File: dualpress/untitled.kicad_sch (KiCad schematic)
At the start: 16 parts, among them J4 Connector, USB-TYPE-C-16P, J5 Connector, USB-TYPE-C-16P

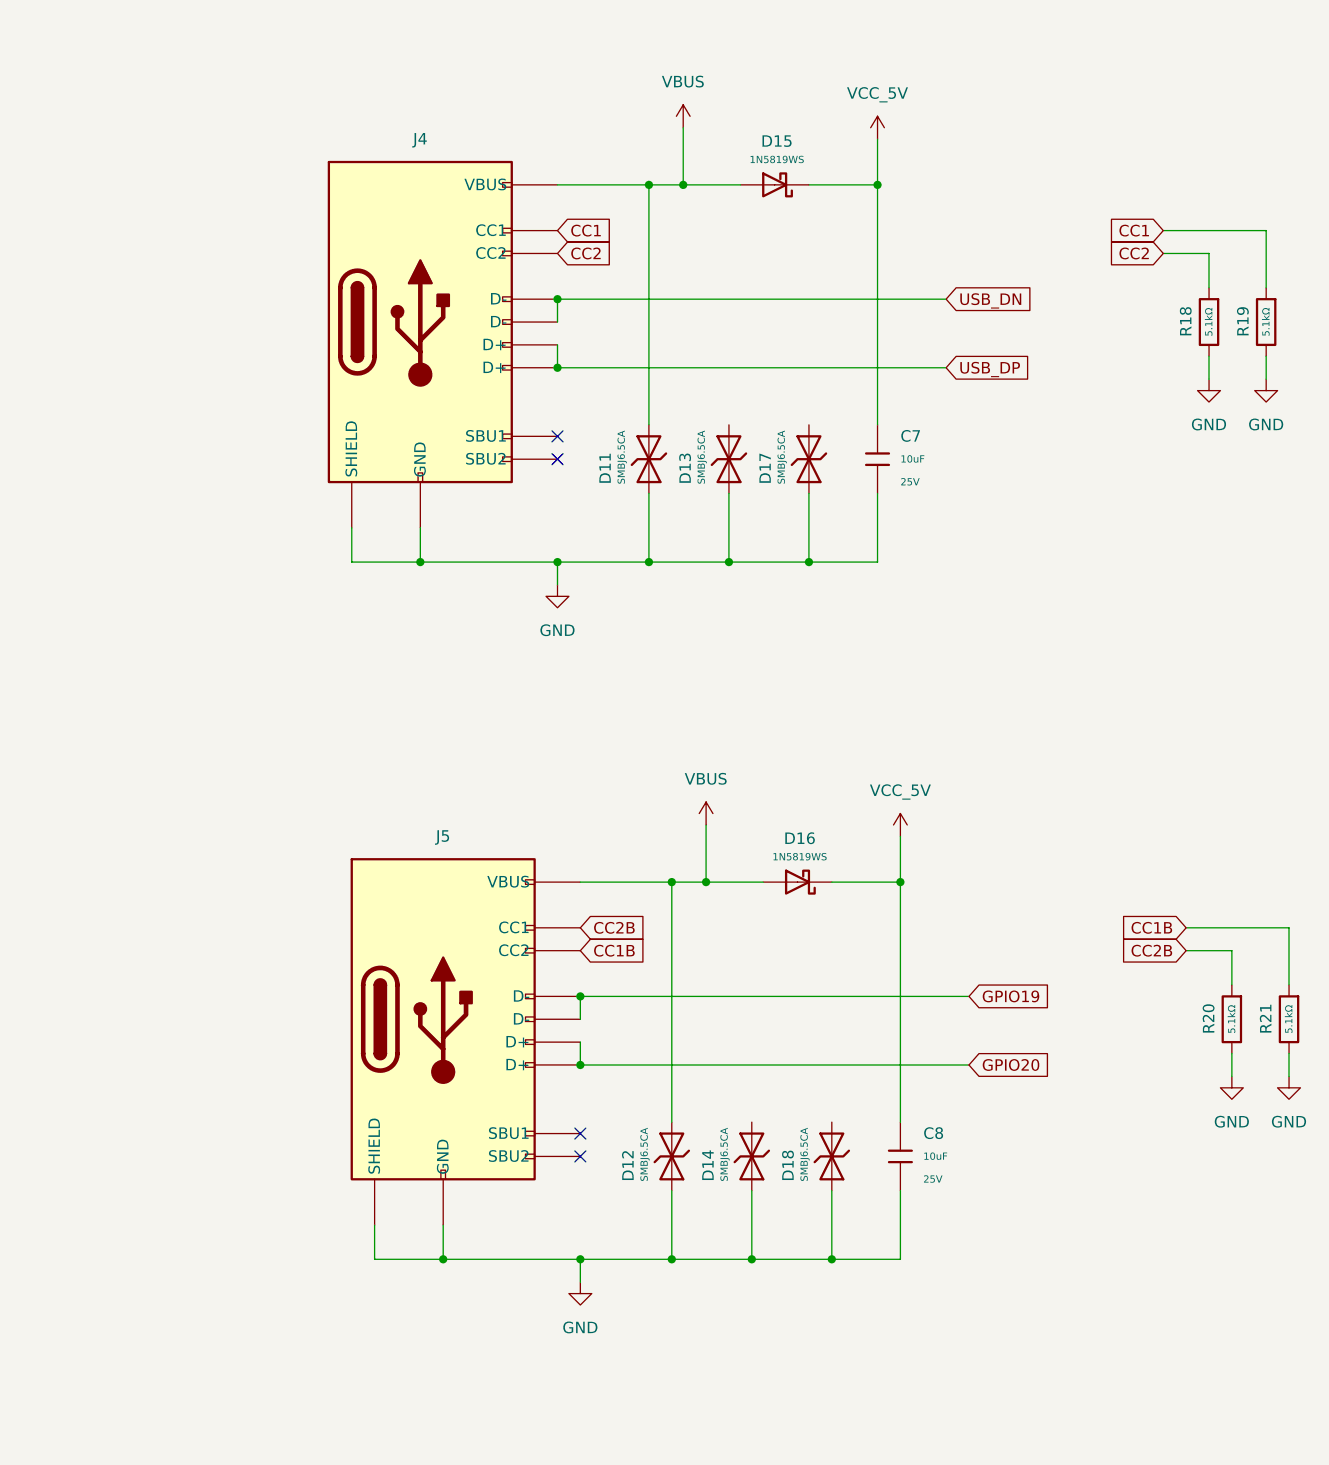
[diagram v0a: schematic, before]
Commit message: schematic done
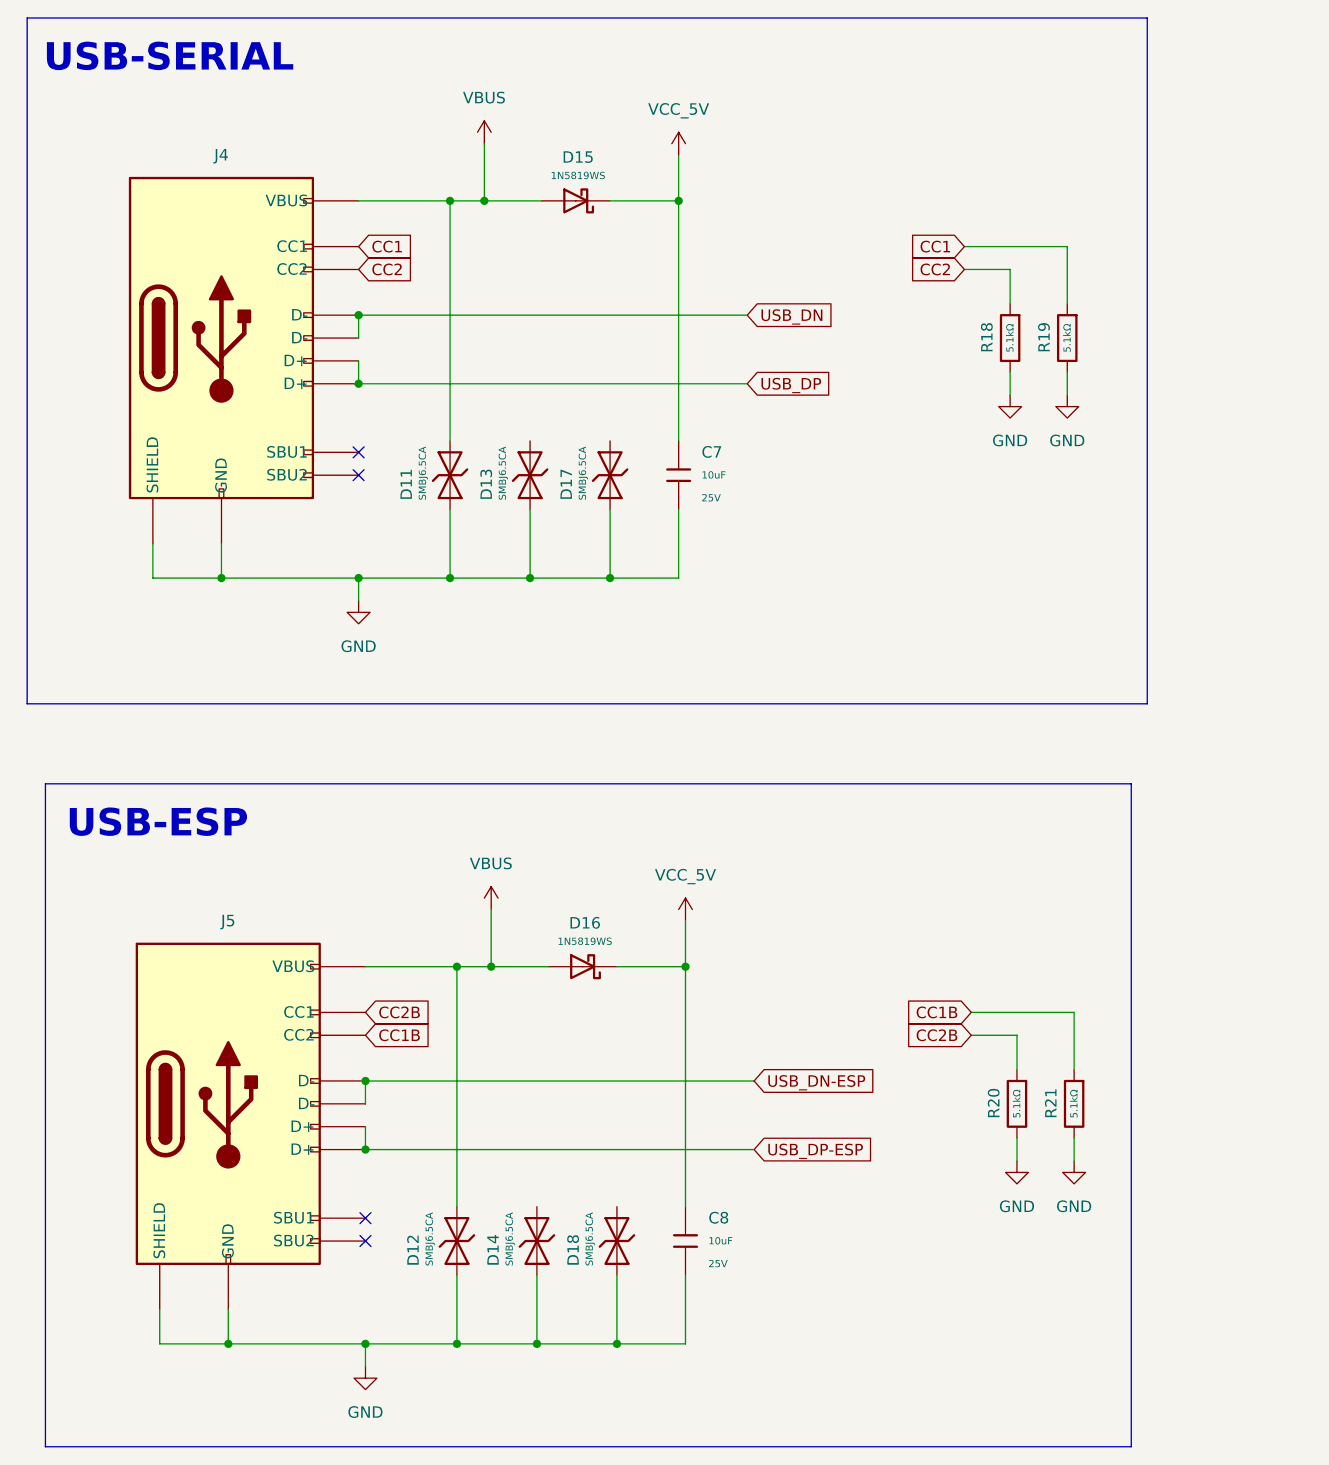
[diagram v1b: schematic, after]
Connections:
- net GPIO19 renamed USB_DN-ESP
- net GPIO20 renamed USB_DP-ESP
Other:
- note added: "USB-ESP"
- note added: "USB-SERIAL"
- moved on the sheet: C7, C8, D11, D12, D13, D14, D15, D16, D17, D18, J4, J5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

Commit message: before remove footprints
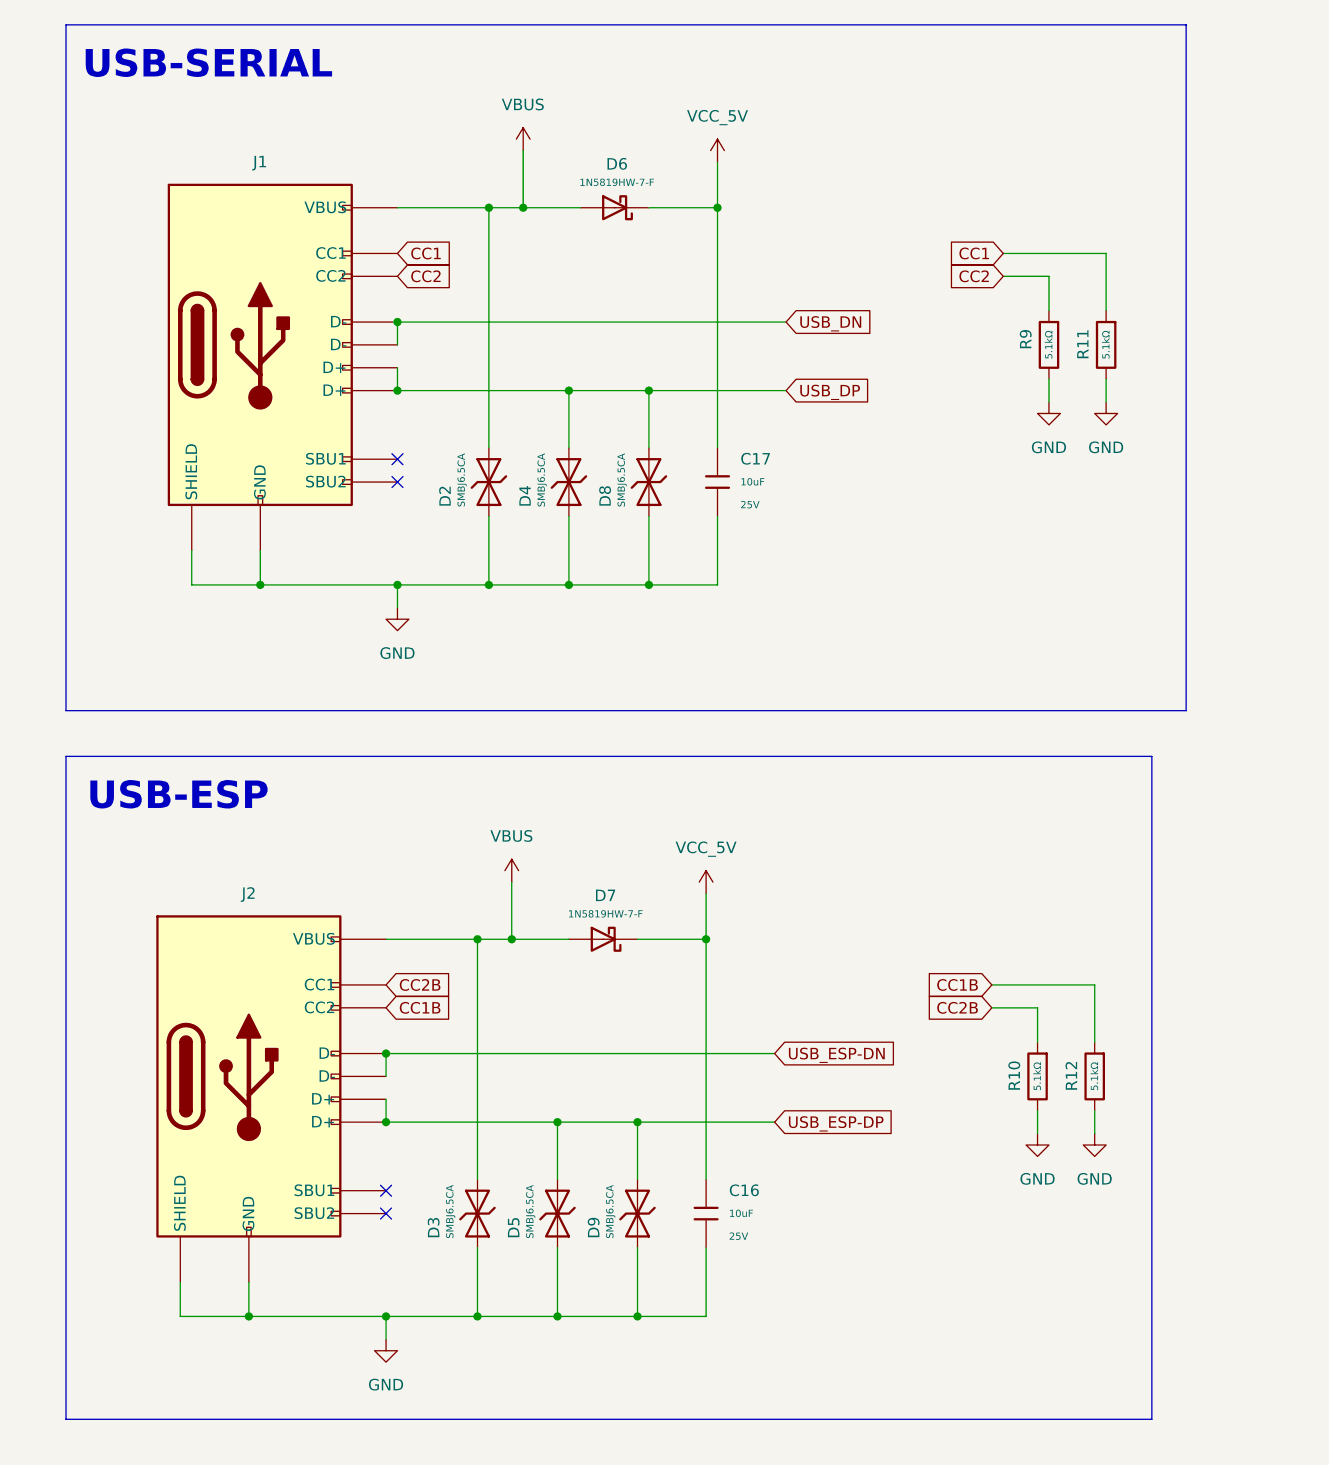
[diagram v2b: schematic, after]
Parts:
- removed C7, C8: 10uF, PCM_JLCPCB:C_0603, symbol PCM_JLCPCB-Capacitors:0603,10uF,(2)
- added C16, C17: 10uF, PCM_JLCPCB:C_0805, symbol PCM_JLCPCB-Capacitors:0805,10uF
- D2: renamed from D11; JLCPCB (none) -> C7420377
- D3: renamed from D12; JLCPCB (none) -> C7420377
- D4: renamed from D13; JLCPCB (none) -> C7420377
- D5: renamed from D14; JLCPCB (none) -> C7420377
- D6: renamed from D15; value 1N5819WS -> 1N5819HW-7-F; footprint PCM_JLCPCB:D_SOD-323 -> PCM_JLCPCB:D_SOD-123; JLCPCB (none) -> C82544; LCSC C191023 -> C82544; Part 1N5819WS -> 1N5819HW-7-F; now left out of the parts list
- D7: renamed from D16; value 1N5819WS -> 1N5819HW-7-F; footprint PCM_JLCPCB:D_SOD-323 -> PCM_JLCPCB:D_SOD-123; JLCPCB (none) -> C82544; now left out of the parts list
- D8: renamed from D17; JLCPCB (none) -> C7420377
- D9: renamed from D18; JLCPCB (none) -> C7420377
- renumbered J4 to J1, J5 to J2, R20 to R10, R19 to R11, R21 to R12, R18 to R9
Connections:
- net USB_DP-ESP is gone; now on net USB_ESP-DP: J2.A6 (D+), J2.B6 (D+)
- net GND: now also C16.2, C17.2
- net USB_DP: now also D4.2, D8.2
- net VCC_5V: now also C16.1, C17.1
- net USB_ESP-DP: now reaches D9.2
- net USB_ESP-DP: now also D5.2
- net USB_DN-ESP renamed USB_ESP-DN
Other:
- moved on the sheet: D2, D3, D4, D5, D6, D7, D8, D9, J1, J2, R10, R11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
